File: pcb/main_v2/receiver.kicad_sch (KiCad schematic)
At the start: 15 parts, among them IC401 RMS-30+, IC402 HMC374, J401 Conn_Coaxial, J402 Conn_Coaxial

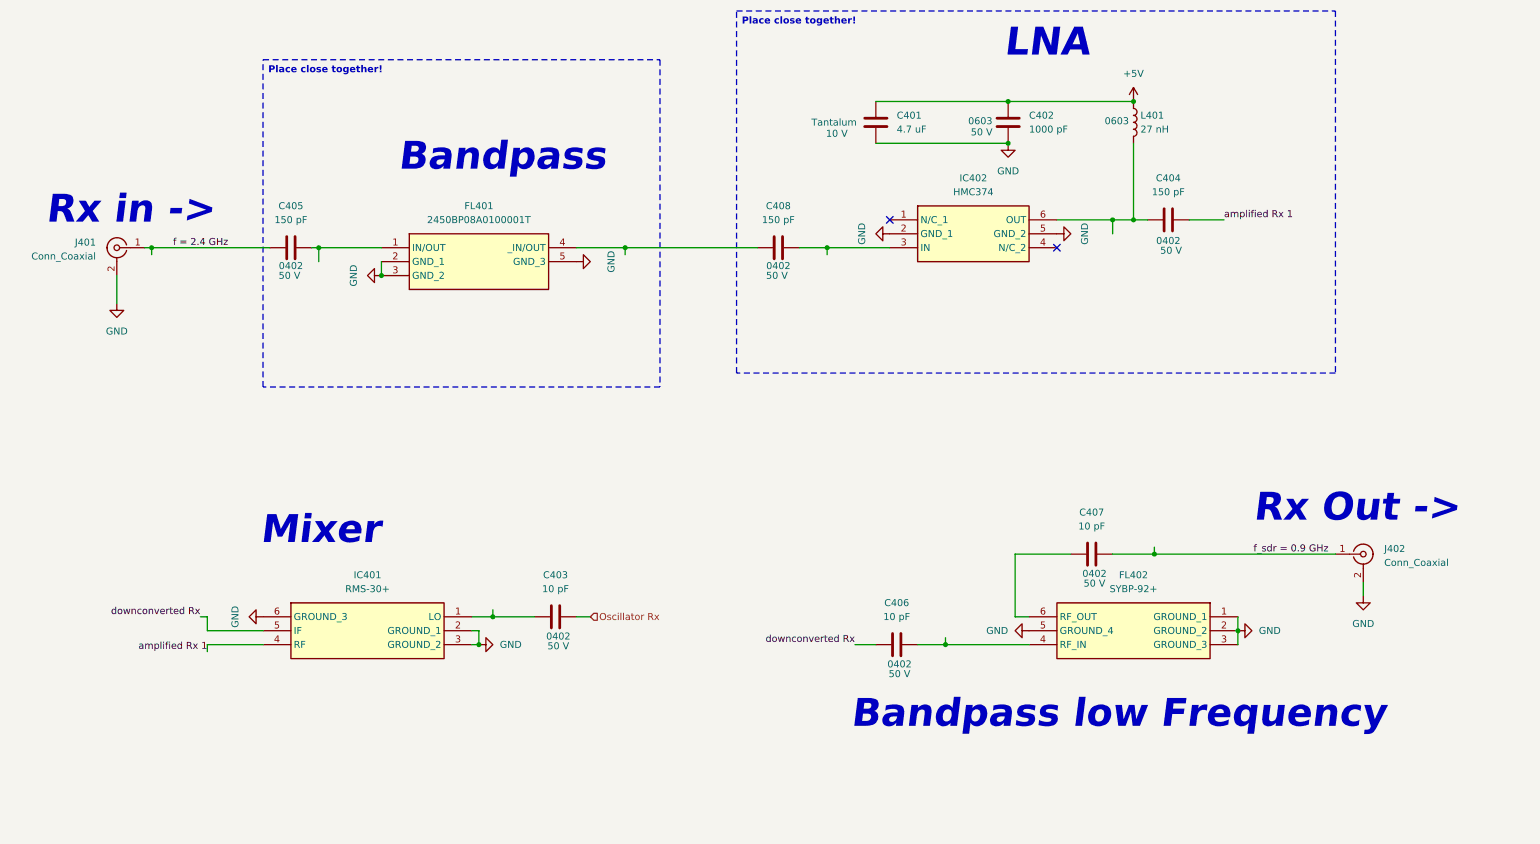
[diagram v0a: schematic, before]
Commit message: updarted schematic and simulation
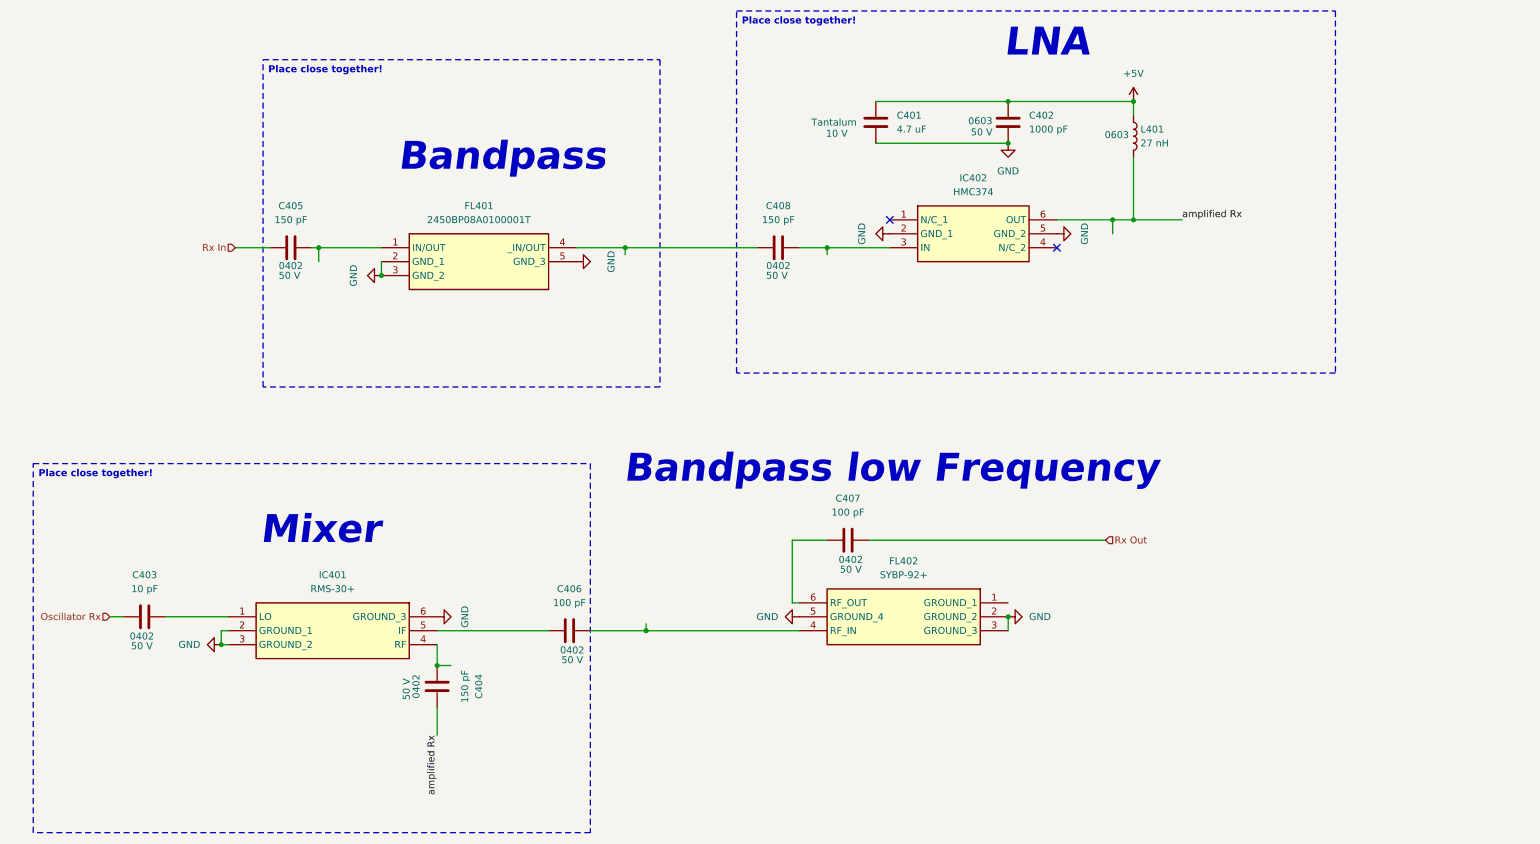
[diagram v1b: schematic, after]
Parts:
- removed J401, J402: Conn_Coaxial, Connector_Coaxial:SMA_Amphenol_132289_EdgeMount, symbol Connector:Conn_Coaxial
- C406, C407: value 10 pF -> 100 pF
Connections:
- net GND: no longer FL402.1 (GROUND_1)
- net amplified Rx: now reaches IC402.6 (OUT), L401.2
- net amplified Rx: now also C404.2; no longer C404.1
- net amplified Rx 1: no longer names the net of IC401.4 (RF)
- net amplified Rx 1: now also C404.1; no longer C404.2
- net downconverted Rx: no longer names the net of C406.1, IC401.5 (IF)
- net f = 2.4 GHz renamed Rx In
- net f_sdr = 0.9 GHz renamed Rx Out
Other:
- note removed: "Rx Out ->"
- note removed: "Rx in ->"
- moved on the sheet: C403, C406, C407, FL402, IC401, L401
